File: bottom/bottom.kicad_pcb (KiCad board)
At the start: 2 copper layers, 27.5 x 37.7 mm, 12 parts, among them P1 HLW4R-2C7LF, P2 BP167911-05340H0A

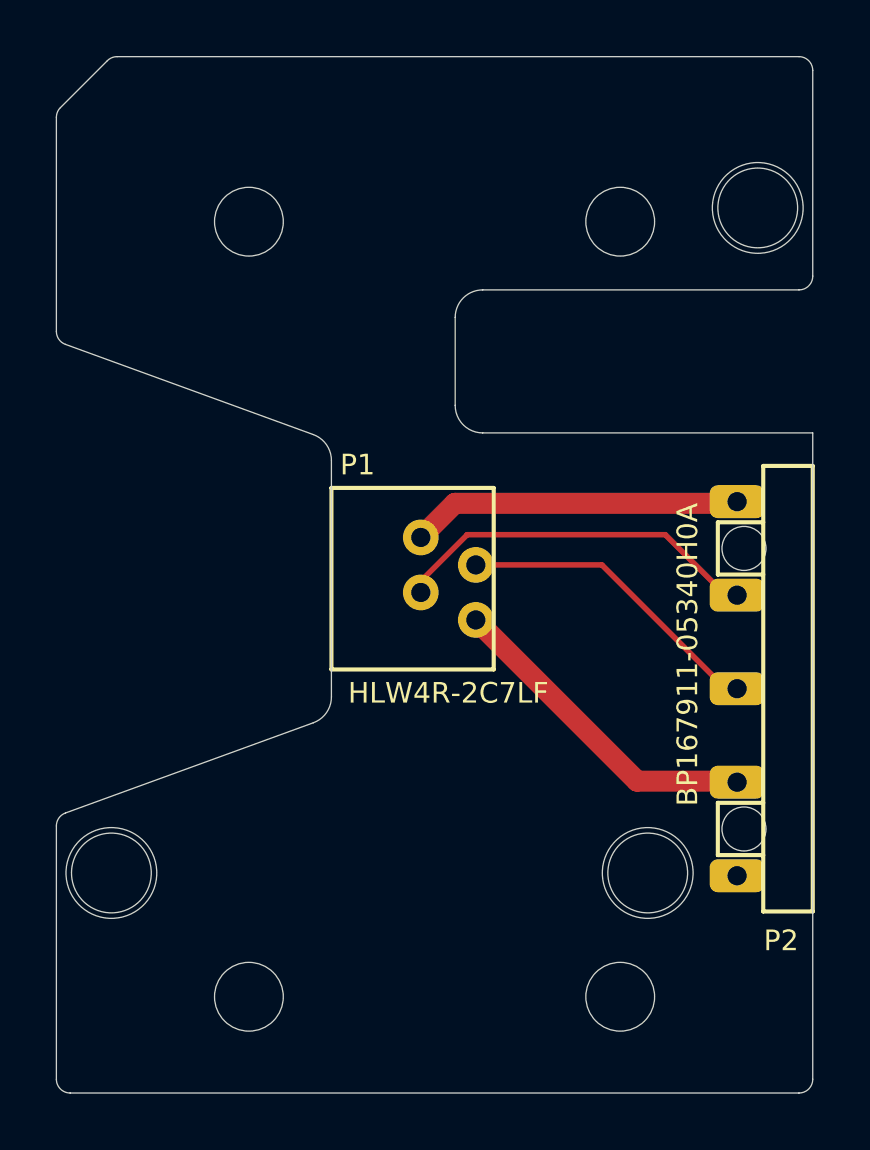
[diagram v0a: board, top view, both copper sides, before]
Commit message: Add UHK logos.
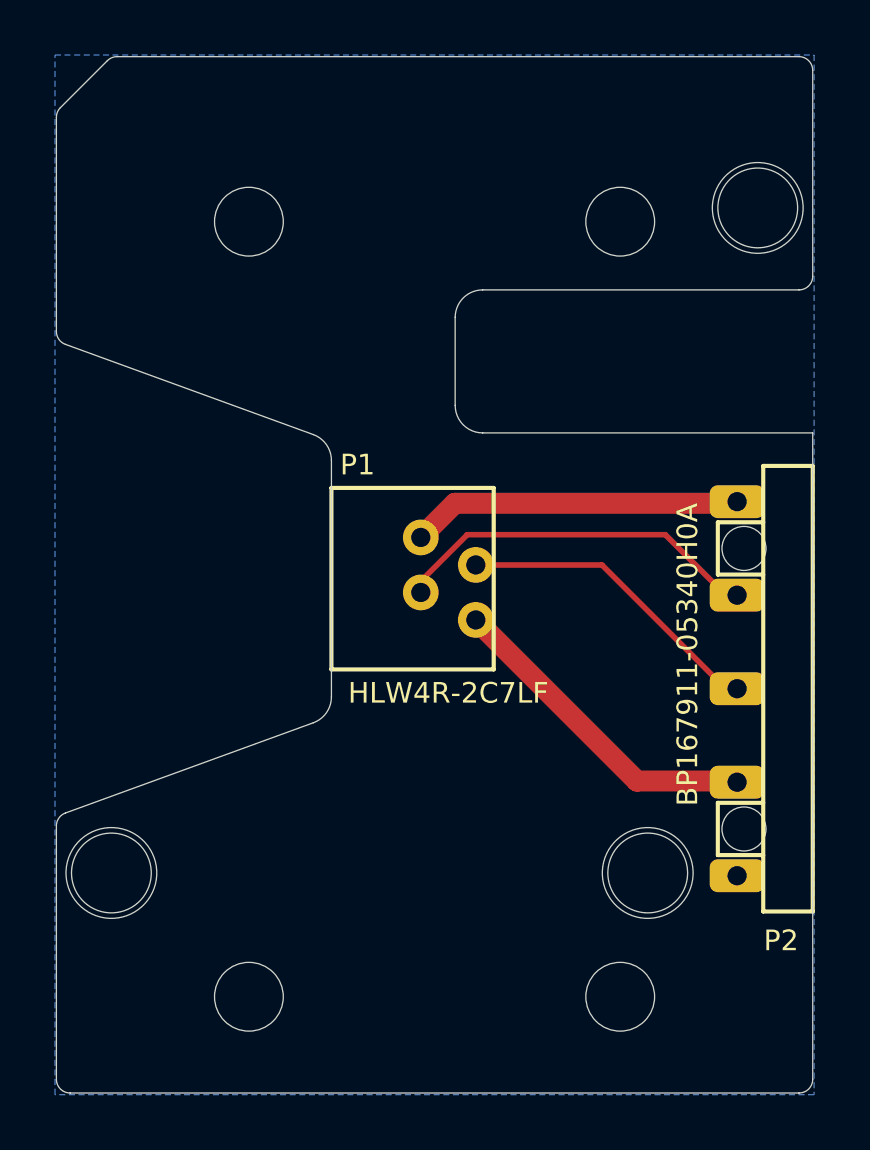
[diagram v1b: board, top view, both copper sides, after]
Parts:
- added G***: LOGO, ugl:UHK_Logo_12x3.4_mm, B.Cu at (209.8, 149.8)
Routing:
- added copper zone on B.Cu, net (none)
